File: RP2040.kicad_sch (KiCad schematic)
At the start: 19 parts, among them U3 RP2040, Y1 12MHz

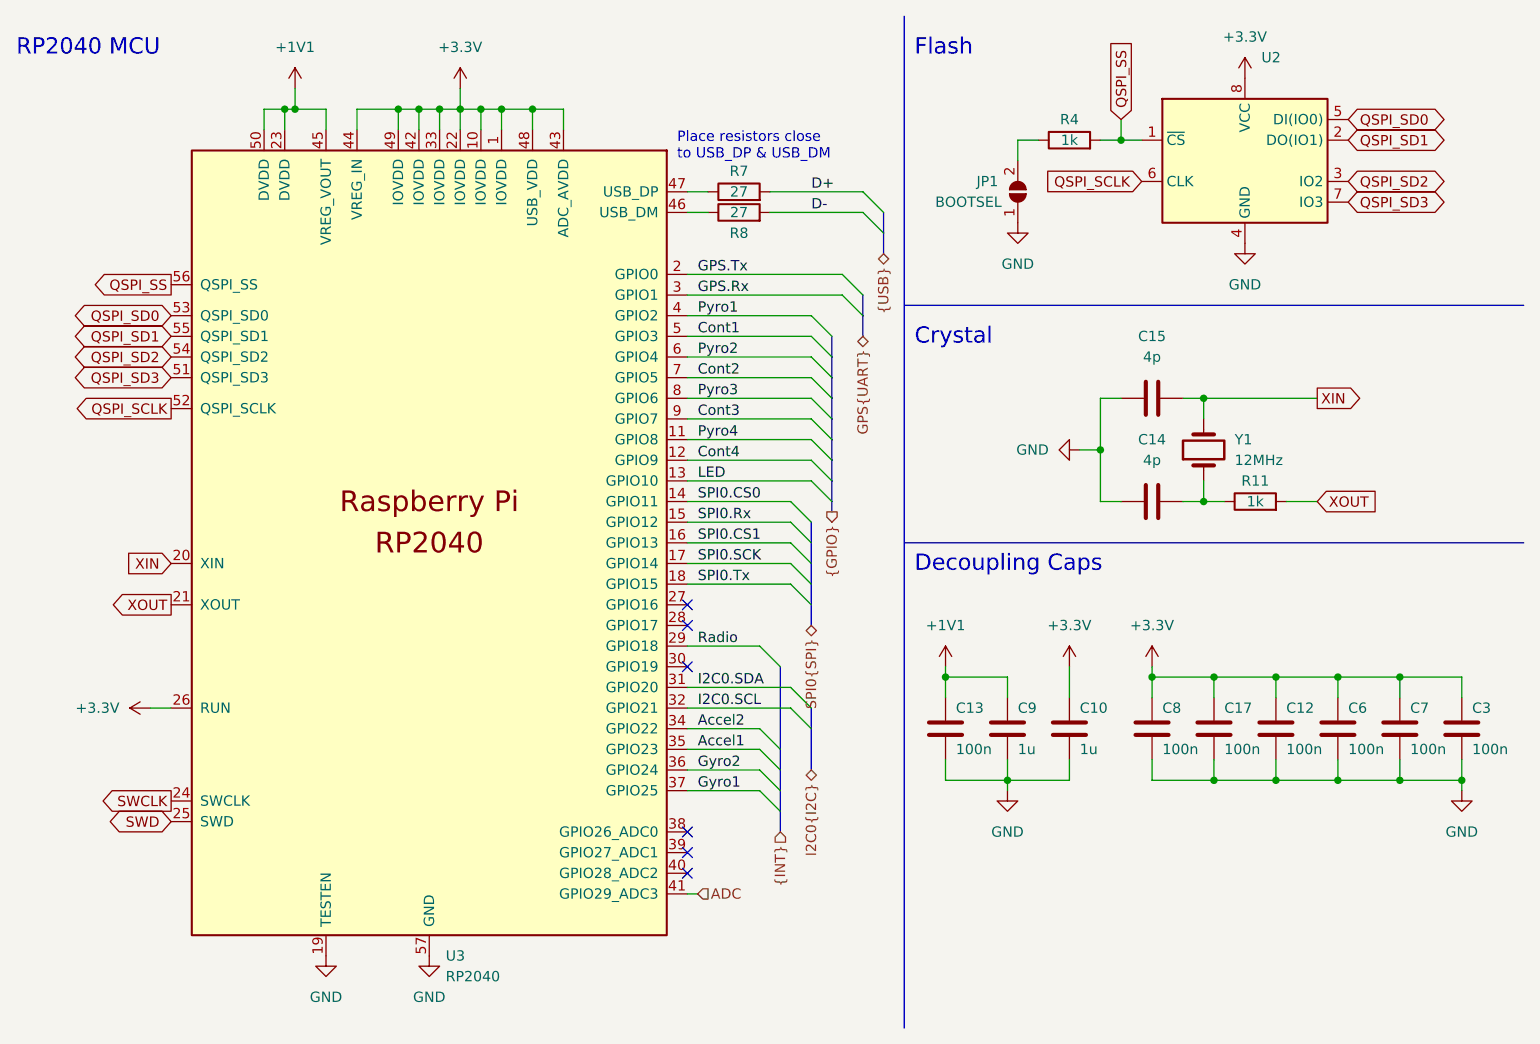
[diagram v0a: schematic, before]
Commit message: Final refinements before issue to JLC
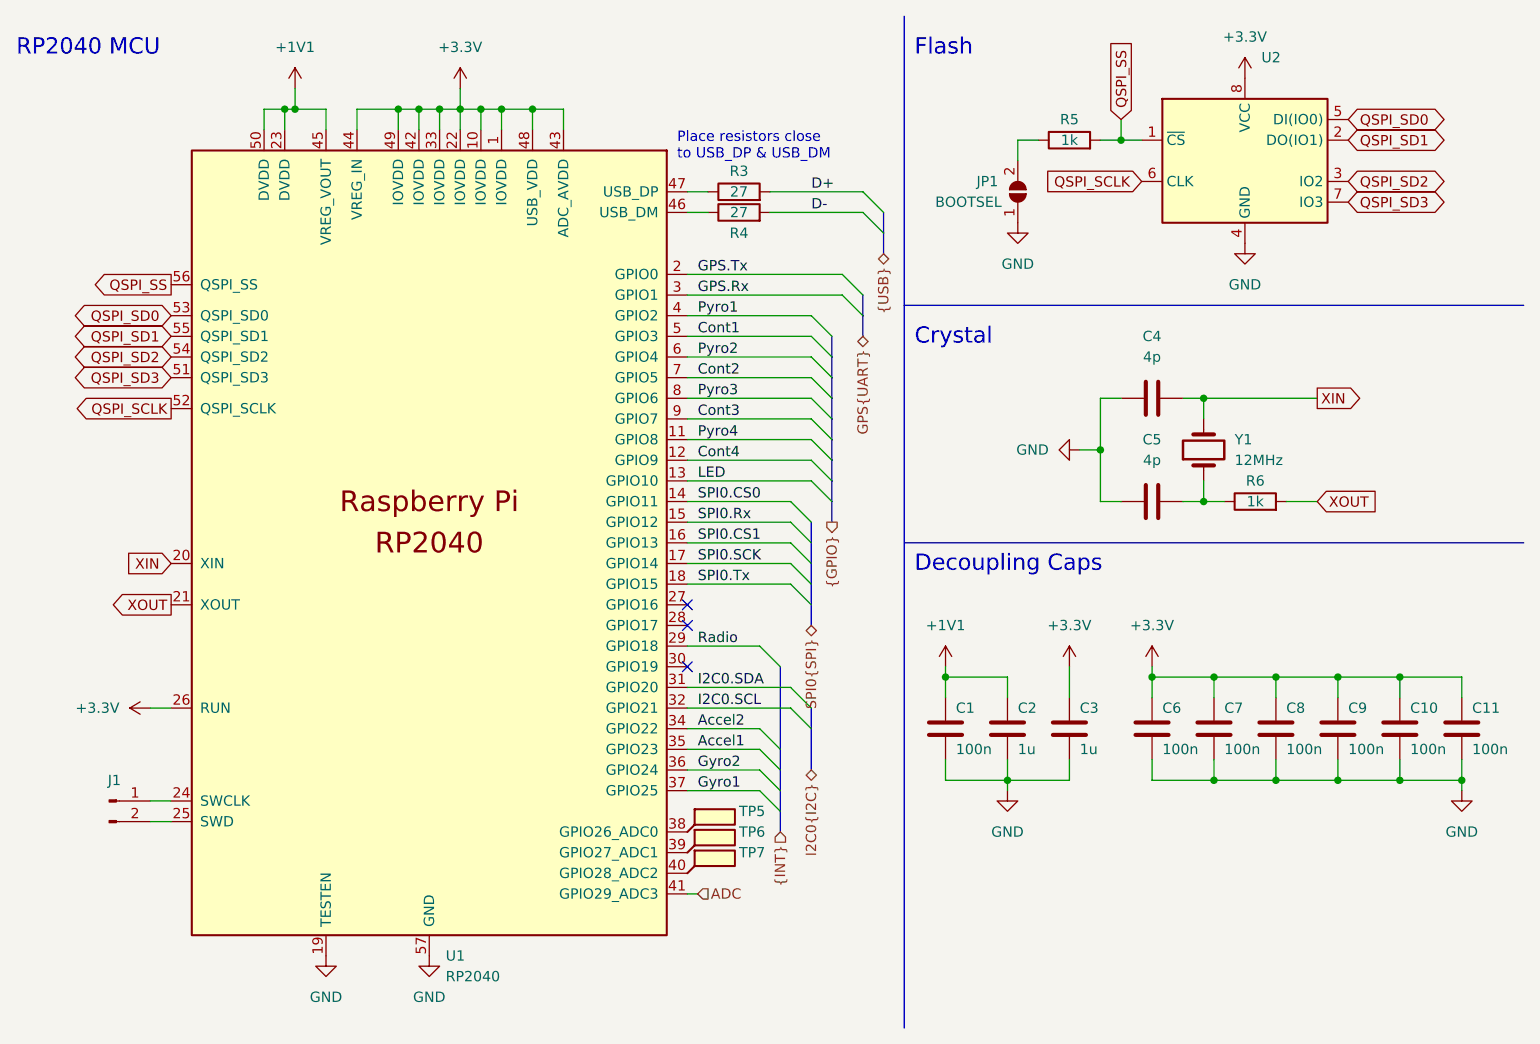
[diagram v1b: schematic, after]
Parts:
- added J1: Conn_01x02_Male, Connector_PinHeader_2.54mm:PinHeader_1x02_P2.54mm_Vertical, symbol Connector:Conn_01x02_Male
- added TP5, TP6, TP7: TestPoint_Flag, TestPoint:TestPoint_Pad_D1.5mm, symbol Connector:TestPoint_Flag
- renumbered C13 to C1, C7 to C10, C3 to C11, C9 to C2, C10 to C3, C15 to C4, C14 to C5, C8 to C6, C17 to C7, C12 to C8, C6 to C9, R7 to R3, R8 to R4, R4 to R5, R11 to R6, U3 to U1
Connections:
- net at U1.38 (GPIO26_ADC0): now also TP5.1
- net at U1.39 (GPIO27_ADC1): now also TP6.1
- net at U1.40 (GPIO28_ADC2): now also TP7.1
- net SWCLK: no longer names the net of U1.24 (SWCLK)
- net SWCLK: now also J1.1 (Pin_1)
- net SWD: no longer names the net of U1.25 (SWD)
- net SWD: now also J1.2 (Pin_2)
- no-connect marks 6 -> 3
